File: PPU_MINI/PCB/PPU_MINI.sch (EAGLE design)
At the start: 92 parts, among them CON1 DIP40, J1 NTSC/PAL, J2 DENDY, J3 PALSEL0, J4 PALSEL1, J5 PALSEL2, J9 BYPASS, T1 BC847, U1 LCMXO2-1200HC, U2 BH7240AKV, U3 SN74LVC8T245, U4 SN74LVC8T245, U5 SN74LVC541A, U6 SN74LVC1G17DBVR, U7 THS7374IPWR, X1 057-010-1

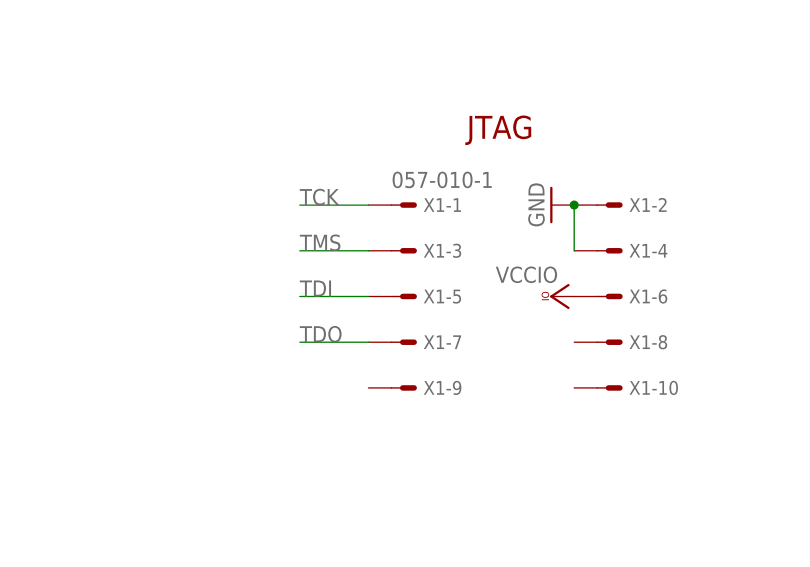
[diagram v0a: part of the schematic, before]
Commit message: Add files via upload
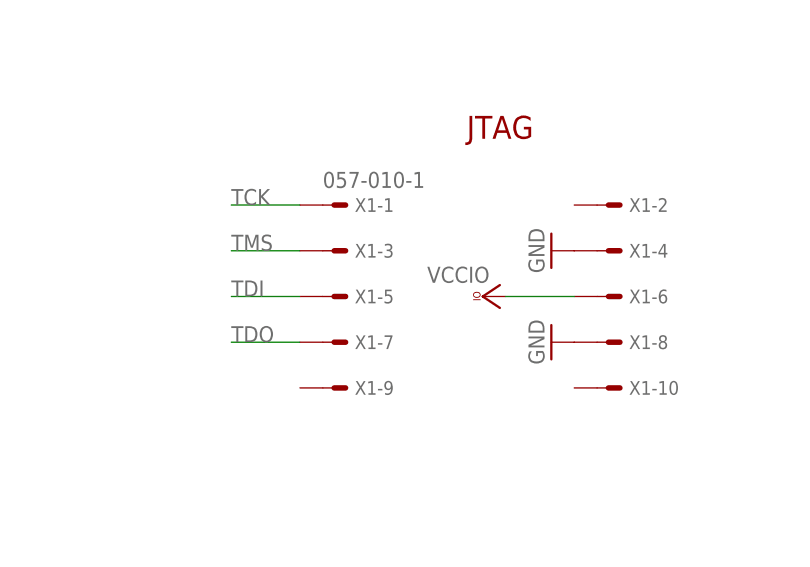
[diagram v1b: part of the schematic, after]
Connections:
- net GND: now also X1-8.S; no longer X1-2.S
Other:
- moved on the sheet: X1-1, X1-3, X1-5, X1-7, X1-9
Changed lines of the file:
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@@
 <part name="GND34" library="supply1" library_urn="urn:adsk.eagle:library:371" deviceset="GND" device=""/>
 <part name="X1" library="con-panduit" library_urn="urn:adsk.eagle:library:169" deviceset="057-010-" device="1" package3d_urn="urn:adsk.eagle:package:9203/1"/>
-<part name="GND43" library="supply1" library_urn="urn:adsk.eagle:library:371" deviceset="GND" device=""/>
 <part name="U3" library="SnapEDA-Library" deviceset="SN74LVC8T245" device=""/>
 <part name="U4" library="SnapEDA-Library" deviceset="SN74LVC8T245" device=""/>
@@
 <part name="VCC2" library="supply1" library_urn="urn:adsk.eagle:library:371" deviceset="VCCIO" device=""/>
 <part name="VCC3" library="supply1" library_urn="urn:adsk.eagle:library:371" deviceset="VCCIO" device=""/>
-<part name="VCC4" library="supply1" library_urn="urn:adsk.eagle:library:371" deviceset="VCCIO" device=""/>
 <part name="VCC5" library="supply1" library_urn="urn:adsk.eagle:library:371" deviceset="VCCIO" device=""/>
 <part name="VCC6" library="supply1" library_urn="urn:adsk.eagle:library:371" deviceset="VCCIO" device=""/>
@@
 <part name="C9" library="rcl_my" deviceset="C-EU" device="C0603" package3d_urn="urn:adsk.eagle:package:23616/2" value="0.1uF"/>
 <part name="C10" library="rcl_my" deviceset="C-EU" device="C0603" package3d_urn="urn:adsk.eagle:package:23616/2" value="0.1uF"/>
+<part name="GND43" library="supply1" library_urn="urn:adsk.eagle:library:371" deviceset="GND" device=""/>
+<part name="GND25" library="supply1" library_urn="urn:adsk.eagle:library:371" deviceset="GND" device=""/>
+<part name="VCC4" library="supply1" library_urn="urn:adsk.eagle:library:371" deviceset="VCCIO" device=""/>
 </parts>
 <sheets>
@@
 <attribute name="VALUE" x="-172.72" y="114.3" size="1.778" layer="96"/>
 </instance>
-<instance part="X1" gate="-1" x="129.54" y="-111.76" smashed="yes">
-<attribute name="NAME" x="130.556" y="-112.522" size="1.524" layer="95"/>
-<attribute name="VALUE" x="127" y="-109.855" size="1.778" layer="96"/>
+<instance part="X1" gate="-1" x="121.92" y="-111.76" smashed="yes">
+<attribute name="NAME" x="122.936" y="-112.522" size="1.524" layer="95"/>
+<attribute name="VALUE" x="119.38" y="-109.855" size="1.778" layer="96"/>
 </instance>
 <instance part="X1" gate="-2" x="152.4" y="-111.76" smashed="yes">
 <attribute name="NAME" x="153.416" y="-112.522" size="1.524" layer="95"/>
 </instance>
-<instance part="X1" gate="-3" x="129.54" y="-116.84" smashed="yes">
-<attribute name="NAME" x="130.556" y="-117.602" size="1.524" layer="95"/>
+<instance part="X1" gate="-3" x="121.92" y="-116.84" smashed="yes">
+<attribute name="NAME" x="122.936" y="-117.602" size="1.524" layer="95"/>
 </instance>
 <instance part="X1" gate="-4" x="152.4" y="-116.84" smashed="yes">
 <attribute name="NAME" x="153.416" y="-117.602" size="1.524" layer="95"/>
 </instance>
-<instance part="X1" gate="-5" x="129.54" y="-121.92" smashed="yes">
-<attribute name="NAME" x="130.556" y="-122.682" size="1.524" layer="95"/>
+<instance part="X1" gate="-5" x="121.92" y="-121.92" smashed="yes">
+<attribute name="NAME" x="122.936" y="-122.682" size="1.524" layer="95"/>
 </instance>
 <instance part="X1" gate="-6" x="152.4" y="-121.92" smashed="yes">
 <attribute name="NAME" x="153.416" y="-122.682" size="1.524" layer="95"/>
 </instance>
-<instance part="X1" gate="-7" x="129.54" y="-127" smashed="yes">
-<attribute name="NAME" x="130.556" y="-127.762" size="1.524" layer="95"/>
+<instance part="X1" gate="-7" x="121.92" y="-127" smashed="yes">
+<attribute name="NAME" x="122.936" y="-127.762" size="1.524" layer="95"/>
 </instance>
 <instance part="X1" gate="-8" x="152.4" y="-127" smashed="yes">
 <attribute name="NAME" x="153.416" y="-127.762" size="1.524" layer="95"/>
 </instance>
-<instance part="X1" gate="-9" x="129.54" y="-132.08" smashed="yes">
-<attribute name="NAME" x="130.556" y="-132.842" size="1.524" layer="95"/>
+<instance part="X1" gate="-9" x="121.92" y="-132.08" smashed="yes">
+<attribute name="NAME" x="122.936" y="-132.842" size="1.524" layer="95"/>
 </instance>
 <instance part="X1" gate="-10" x="152.4" y="-132.08" smashed="yes">
 <attribute name="NAME" x="153.416" y="-132.842" size="1.524" layer="95"/>
-</instance>
-<instance part="GND43" gate="1" x="144.78" y="-111.76" smashed="yes" rot="R270">
-<attribute name="VALUE" x="142.24" y="-109.22" size="1.778" layer="96" rot="R270"/>
 </instance>
 <instance part="U3" gate="G$1" x="-147.32" y="-12.7" smashed="yes">
@@
 <attribute name="VALUE" x="-42.418" y="51.562" size="1.778" layer="96" rot="R180"/>
 </instance>
-<instance part="VCC4" gate="G$1" x="144.78" y="-121.92" smashed="yes" rot="R90">
-<attribute name="VALUE" x="145.542" y="-118.618" size="1.778" layer="96" rot="R180"/>
-</instance>
 <instance part="VCC5" gate="G$1" x="-91.44" y="-30.48" smashed="yes" rot="R90">
 <attribute name="VALUE" x="-93.218" y="-29.718" size="1.778" layer="96" rot="R180"/>
@@
 <attribute name="NAME" x="-175.26" y="-60.071" size="1.778" layer="95" rot="R180"/>
 <attribute name="VALUE" x="-172.974" y="-65.151" size="1.778" layer="96" rot="R180"/>
+</instance>
+<instance part="GND43" gate="1" x="144.78" y="-116.84" smashed="yes" rot="R270">
+<attribute name="VALUE" x="142.24" y="-114.3" size="1.778" layer="96" rot="R270"/>
+</instance>
+<instance part="GND25" gate="1" x="144.78" y="-127" smashed="yes" rot="R270">
+<attribute name="VALUE" x="142.24" y="-124.46" size="1.778" layer="96" rot="R270"/>
+</instance>
+<instance part="VCC4" gate="G$1" x="137.16" y="-121.92" smashed="yes" rot="R90">
+<attribute name="VALUE" x="137.922" y="-118.618" size="1.778" layer="96" rot="R180"/>
 </instance>
 </instances>
@@
 <segment>
 <pinref part="X1" gate="-1" pin="S"/>
-<wire x1="124.46" y1="-111.76" x2="116.84" y2="-111.76" width="0.1524" layer="91"/>
-<label x="116.84" y="-111.76" size="1.778" layer="95"/>
+<wire x1="116.84" y1="-111.76" x2="109.22" y2="-111.76" width="0.1524" layer="91"/>
+<label x="109.22" y="-111.76" size="1.778" layer="95"/>
 </segment>
 <segment>
@@
 </net>
 <net name="GND" class="0">
-<segment>
-<pinref part="X1" gate="-2" pin="S"/>
-<pinref part="GND43" gate="1" pin="GND"/>
-<pinref part="X1" gate="-4" pin="S"/>
-<wire x1="147.32" y1="-116.84" x2="147.32" y2="-111.76" width="0.1524" layer="91"/>
-<junction x="147.32" y="-111.76"/>
-</segment>
 <segment>
 <pinref part="GND6" gate="1" pin="GND"/>
@@
 <pinref part="GND38" gate="1" pin="GND"/>
 </segment>
+<segment>
+<pinref part="GND25" gate="1" pin="GND"/>
+<pinref part="X1" gate="-8" pin="S"/>
+</segment>
+<segment>
+<pinref part="X1" gate="-4" pin="S"/>
+<pinref part="GND43" gate="1" pin="GND"/>
+</segment>
 </net>
 <net name="TDI" class="0">
@@
 </segment>
 <segment>
-<wire x1="124.46" y1="-121.92" x2="116.84" y2="-121.92" width="0.1524" layer="91"/>
+<wire x1="116.84" y1="-121.92" x2="109.22" y2="-121.92" width="0.1524" layer="91"/>
 <pinref part="X1" gate="-5" pin="S"/>
-<label x="116.84" y="-121.92" size="1.778" layer="95"/>
+<label x="109.22" y="-121.92" size="1.778" layer="95"/>
 </segment>
 </net>
@@
 </segment>
 <segment>
-<wire x1="124.46" y1="-116.84" x2="116.84" y2="-116.84" width="0.1524" layer="91"/>
+<wire x1="116.84" y1="-116.84" x2="109.22" y2="-116.84" width="0.1524" layer="91"/>
 <pinref part="X1" gate="-3" pin="S"/>
-<label x="116.84" y="-116.84" size="1.778" layer="95"/>
+<label x="109.22" y="-116.84" size="1.778" layer="95"/>
 </segment>
 </net>
@@
 </segment>
 <segment>
-<wire x1="124.46" y1="-127" x2="116.84" y2="-127" width="0.1524" layer="91"/>
+<wire x1="116.84" y1="-127" x2="109.22" y2="-127" width="0.1524" layer="91"/>
 <pinref part="X1" gate="-7" pin="S"/>
-<label x="116.84" y="-127" size="1.778" layer="95"/>
+<label x="109.22" y="-127" size="1.778" layer="95"/>
 </segment>
 </net>
@@
 <pinref part="R21" gate="G$1" pin="1"/>
 <pinref part="C29" gate="G$1" pin="2"/>
-<pinref part="R22" gate="G$1" pin="2"/>
 <pinref part="R22" gate="G$1" pin="2"/>
 <junction x="119.38" y="111.76"/>
@@
 </segment>
 <segment>
+<pinref part="VCC4" gate="G$1" pin="VCCIO"/>
 <pinref part="X1" gate="-6" pin="S"/>
-<pinref part="VCC4" gate="G$1" pin="VCCIO"/>
-</segment>
-</net>
+<wire x1="139.7" y1="-121.92" x2="147.32" y2="-121.92" width="0.1524" layer="91"/>
+</segment>
+</net>
